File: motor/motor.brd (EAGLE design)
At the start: 59.7 x 53.3 mm, 3 parts

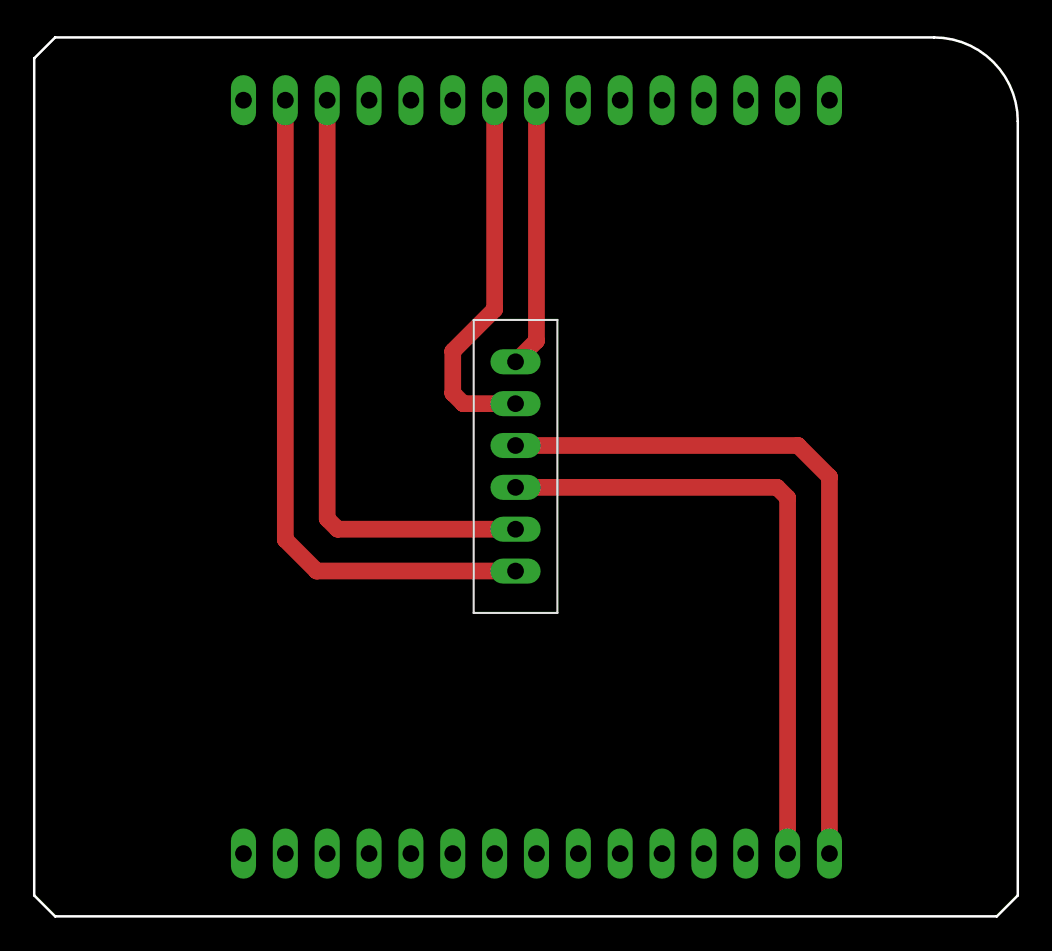
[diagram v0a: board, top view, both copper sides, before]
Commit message: Added breadboard board. This commit is going to production.
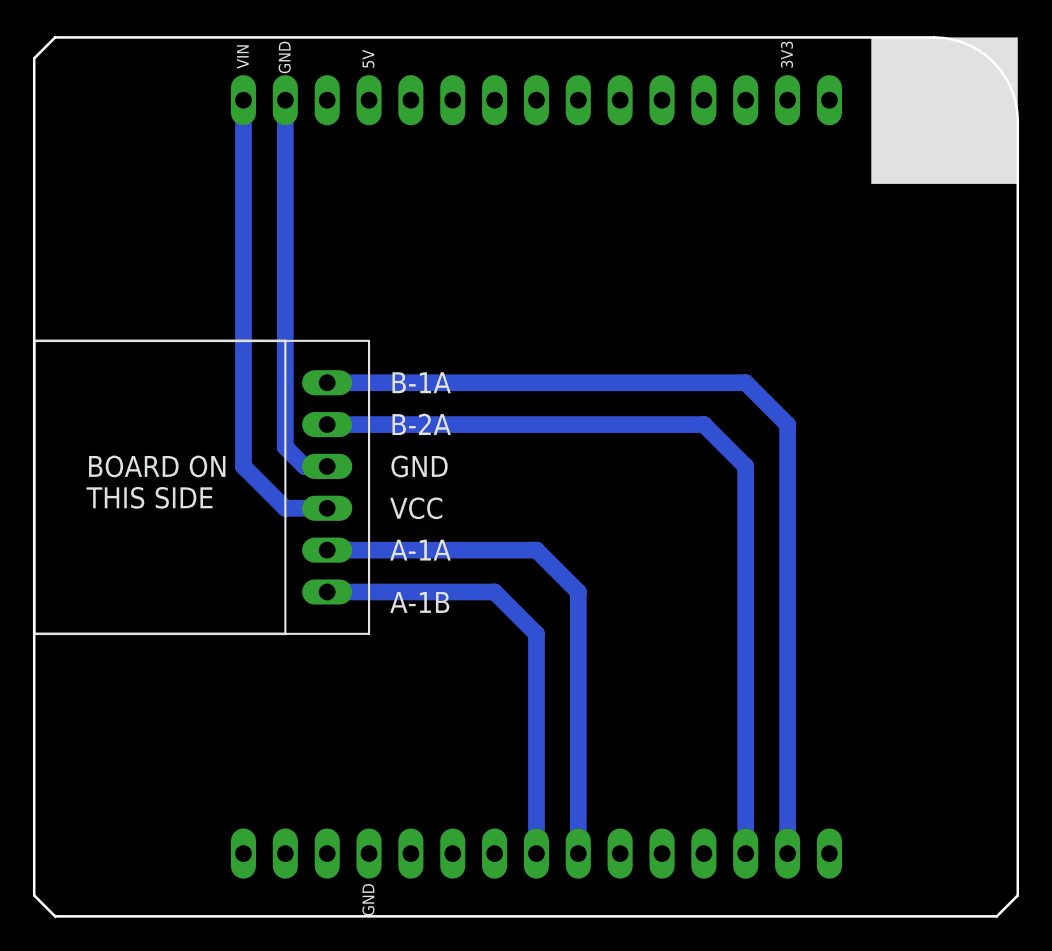
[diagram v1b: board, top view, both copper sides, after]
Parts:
- moved U$1 45.7 mm to (30.5, 3.81), turned to 180 degrees
- moved U$7 45.7 mm to (30.5, 49.5), turned to 180 degrees
- moved U$2 12.0 mm to (17.8, 24.8), turned to 270 degrees
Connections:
- net N$1 renamed GND
- net N$2 renamed VIN
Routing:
- net VIN: track 42.7 -> 28.4 mm
- net GND: track 38.4 -> 24.1 mm
- net N$3: track 41.4 -> 55.0 mm
- net N$4: track 37.1 -> 49.9 mm
- net D05: track 16.4 -> 27.1 mm
- net D06: track 22.9 -> 32.2 mm
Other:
- board text added: "3V3"
- board text added: "5V"
- board text added: "A-1A"
- board text added: "A-1B"
- board text added: "B-1A"
- board text added: "B-2A"
- board text added: "BOARD ON THIS SIDE"
- board text added: "GND"
- board text added: "RC CARS MOTOR BOARD v0.1"
- board text added: "VCC"
- board text added: "VIN"
